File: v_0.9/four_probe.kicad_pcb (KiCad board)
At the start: 2 copper layers, 79 parts, among them J1 Conn_01x26_Male, J2 RG, J3 CONSMA001-SMD-G, J4 CONSMA001-SMD-G, J5 CONSMA001-SMD-G, J6 CONSMA001-SMD-G, U1 LMC6482, U10 ADG704, U11 tmux1511, U2 AD623, U3 LMC6482, U4 AD623, U5 LMC6484, U6 LMC6484, U7 tmux1511, U8 ADG704, U9 ADG704

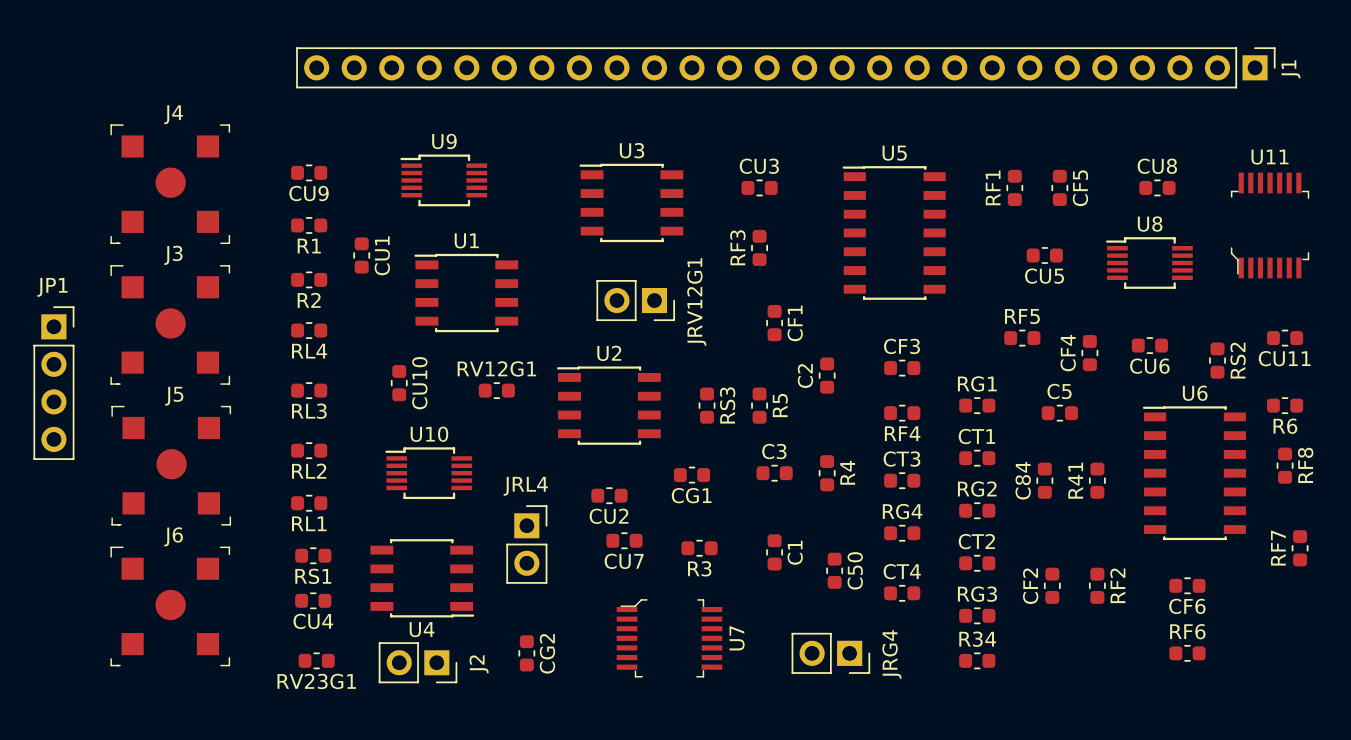
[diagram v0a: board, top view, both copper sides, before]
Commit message: update
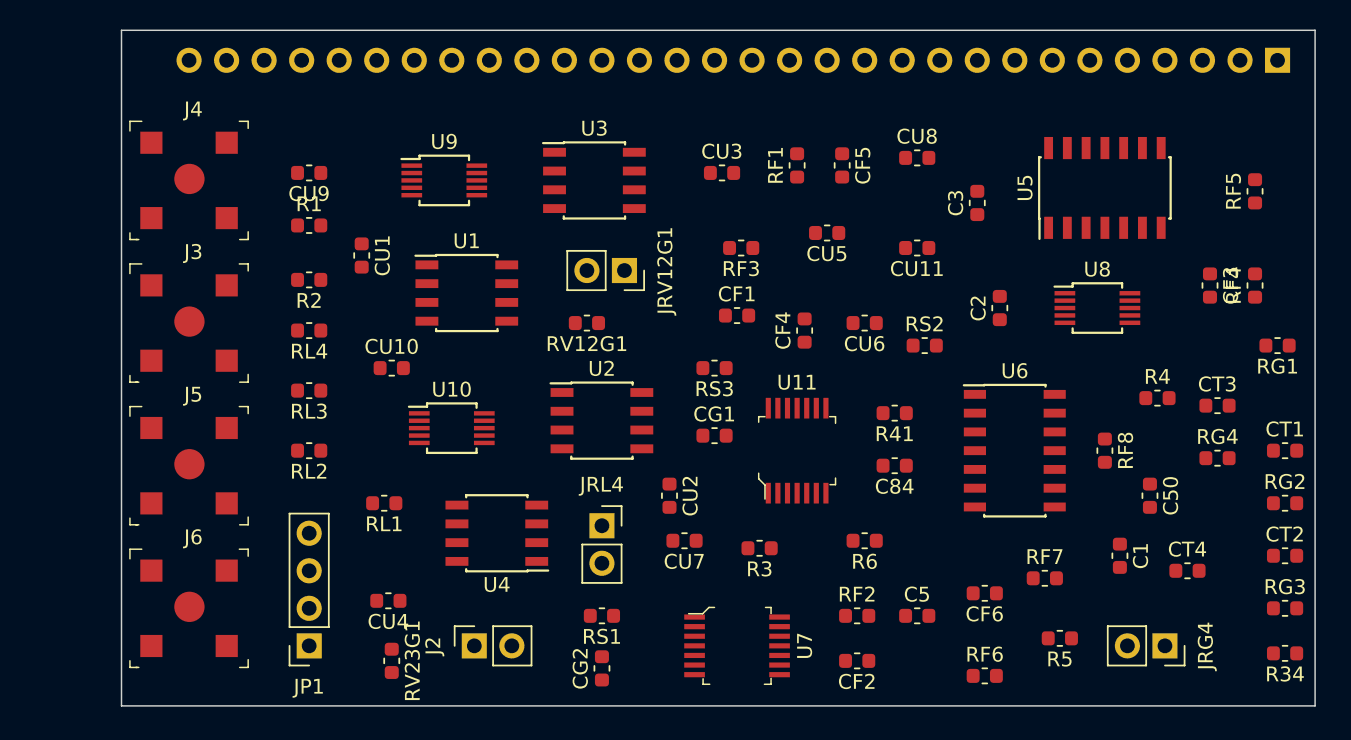
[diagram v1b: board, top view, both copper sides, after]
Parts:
- J1: value Conn_01x26_Male -> Conn_01x30_Male; footprint Connector_PinHeader_2.54mm:PinHeader_1x26_P2.54mm_Vertical -> Connector_PinHeader_2.54mm:PinHeader_1x30_P2.54mm_Vertical; moved to B.Cu
- moved U11 35.4 mm to (103.6, 131.1)
- moved R6 29.9 mm to (108.2, 137.2)
- moved JP1 27.6 mm to (70.6, 144.3), turned to 180 degrees
- moved R5 25.7 mm to (121.4, 143.8), turned to 180 degrees
- moved CU11 25.6 mm to (111.8, 117.3)
- moved RF4 25.4 mm to (134.6, 119.9), turned to 90 degrees
- moved C1 23.4 mm to (125.5, 138.2)
- moved R4 22.9 mm to (128.0, 127.5), turned to 0 degrees
- moved C3 22.9 mm to (115.8, 114.3), turned to 90 degrees
- moved CT3 21.9 mm to (132.1, 128.0)
- moved RG4 21.9 mm to (132.1, 131.6)
- moved C50 21.9 mm to (127.5, 134.1)
- moved CF3 21.6 mm to (131.6, 119.9), turned to 270 degrees
- moved JRG4 21.3 mm to (128.5, 144.3)
- moved CT1 20.8 mm to (136.7, 131.1)
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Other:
- board outline added: 80.8 x 45.7 mm
